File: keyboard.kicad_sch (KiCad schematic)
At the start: 27 parts, among them J1 USB_C_Receptacle_USB2.0_14P, SW1 SW_Push, SW2 SW_Push, SW3 SW_Push, SW4 SW_Push, SW5 SW_Push, U1 ATmega32U4-A, Y1 Crystal_GND24_Small

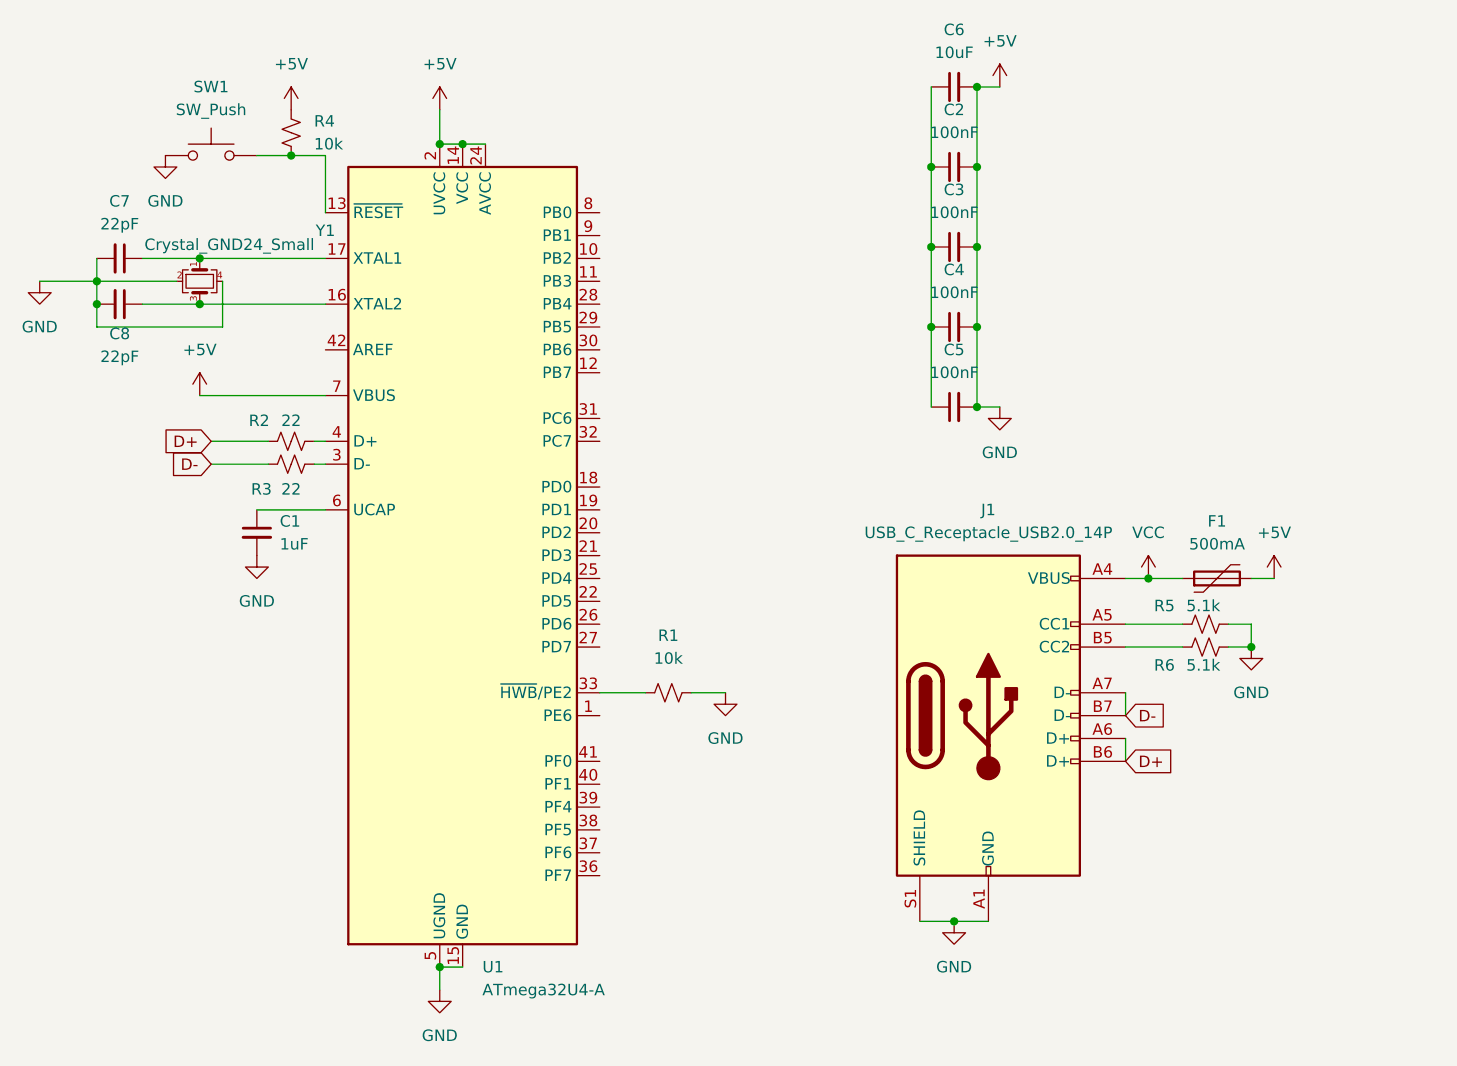
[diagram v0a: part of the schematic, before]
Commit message: bad
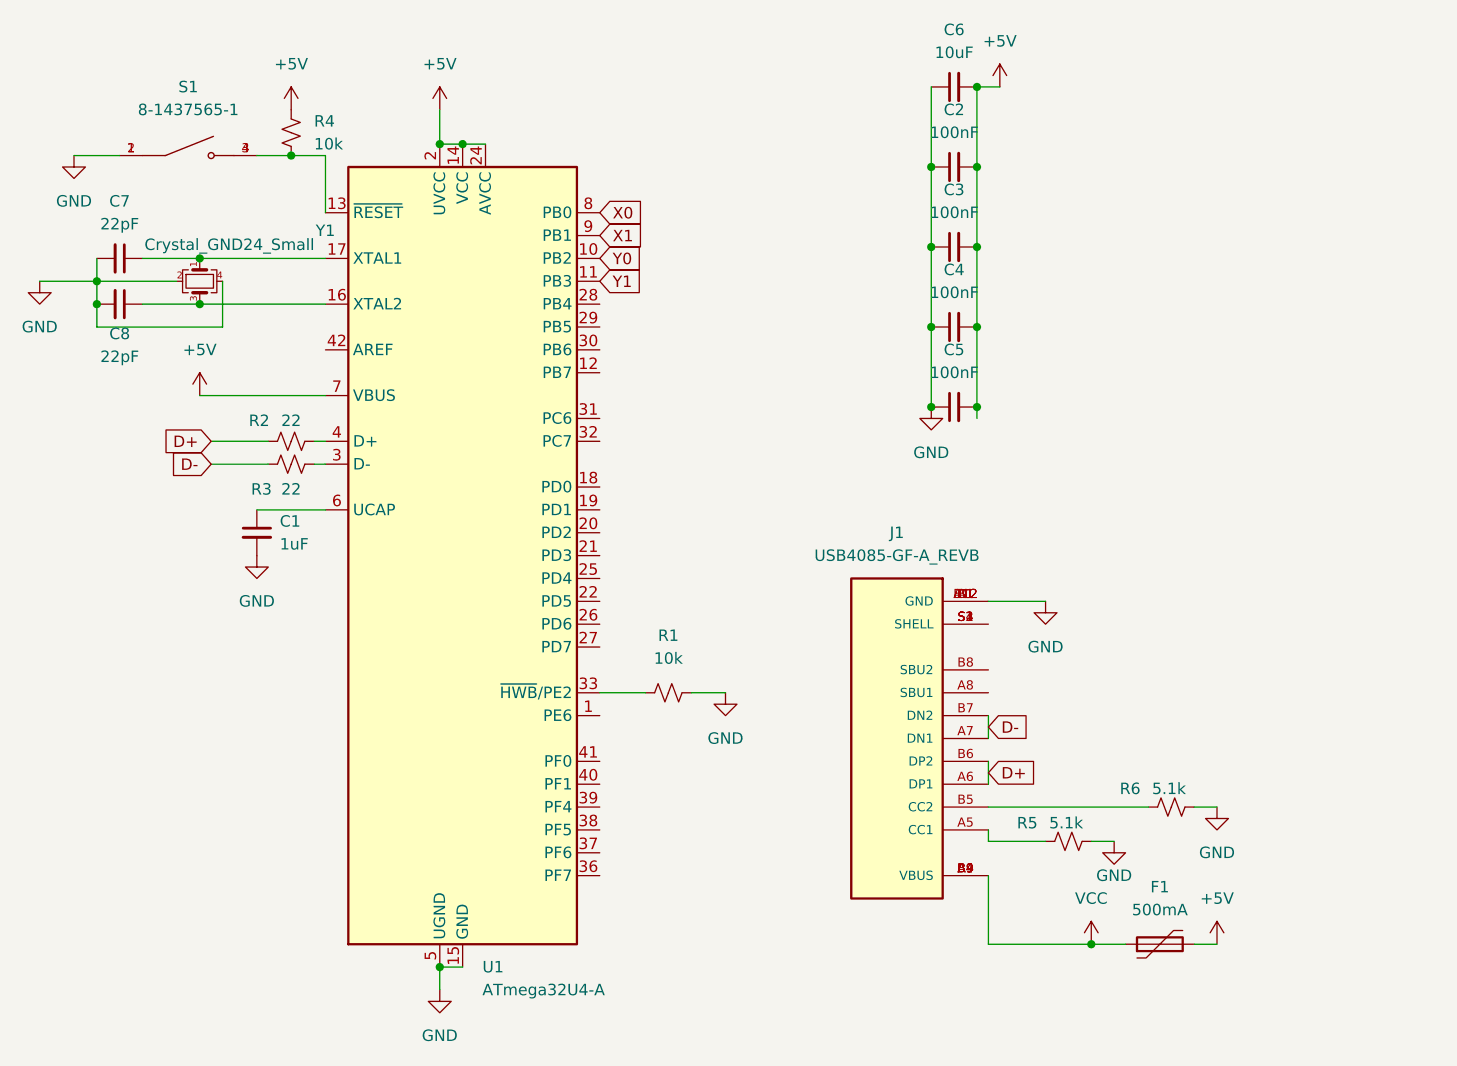
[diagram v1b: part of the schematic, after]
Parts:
- removed J1: USB_C_Receptacle_USB2.0_14P, symbol Connector:USB_C_Receptacle_USB2.0_14P
- removed SW1: SW_Push, symbol Switch:SW_Push
- added J1: USB4085-GF-A_REVB, USB-C:GCT_USB4085-GF-A_REVB, symbol USB4085-GF-A_REVB:USB4085-GF-A_REVB
- added S1: 8-1437565-1, Button:SW_8-1437565-1, symbol 8-1437565-1:8-1437565-1
- SW2, SW3, SW4, SW5: footprint (none) -> MX_keys:MX-Hotswap-1U
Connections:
- net +5V: no longer C1.2, C7.2, C8.2, R1.2, R5.2, R6.2, U1.15 (GND), U1.23 (GND), U1.35 (GND), U1.43 (GND), U1.5 (UGND), Y1.2, Y1.4
- net D+: now also J1.A6 (DP1), J1.B6 (DP2)
- net D-: now also J1.A7 (DN1), J1.B7 (DN2)
- net VCC: now also J1.A4 (VBUS), J1.A9 (VBUS), J1.B4 (VBUS), J1.B9 (VBUS)
- net X0: now also U1.8 (PB0)
- net X1: now also U1.9 (PB1)
- net Y0: now also U1.10 (PB2)
- net Y1: now also U1.11 (PB3)
- net at R4.2, U1.13 (~{RESET}): now also S1.3, S1.4
- net GND: now reaches C2.1, C3.1, C4.1, C5.1, C6.1
- net GND: now also C1.2, C7.2, C8.2, R1.2, R5.2, R6.2, U1.15 (GND), U1.23 (GND), U1.35 (GND), U1.43 (GND), U1.5 (UGND), Y1.2, Y1.4, J1.A1 (GND), J1.A12 (GND), J1.B1 (GND), J1.B12 (GND), S1.1, S1.2
- net at R6.1: now also J1.B5 (CC2)
- net at R5.1: now also J1.A5 (CC1)
- new net: J1.S1 (SHELL), J1.S2 (SHELL), J1.S3 (SHELL), J1.S4 (SHELL)

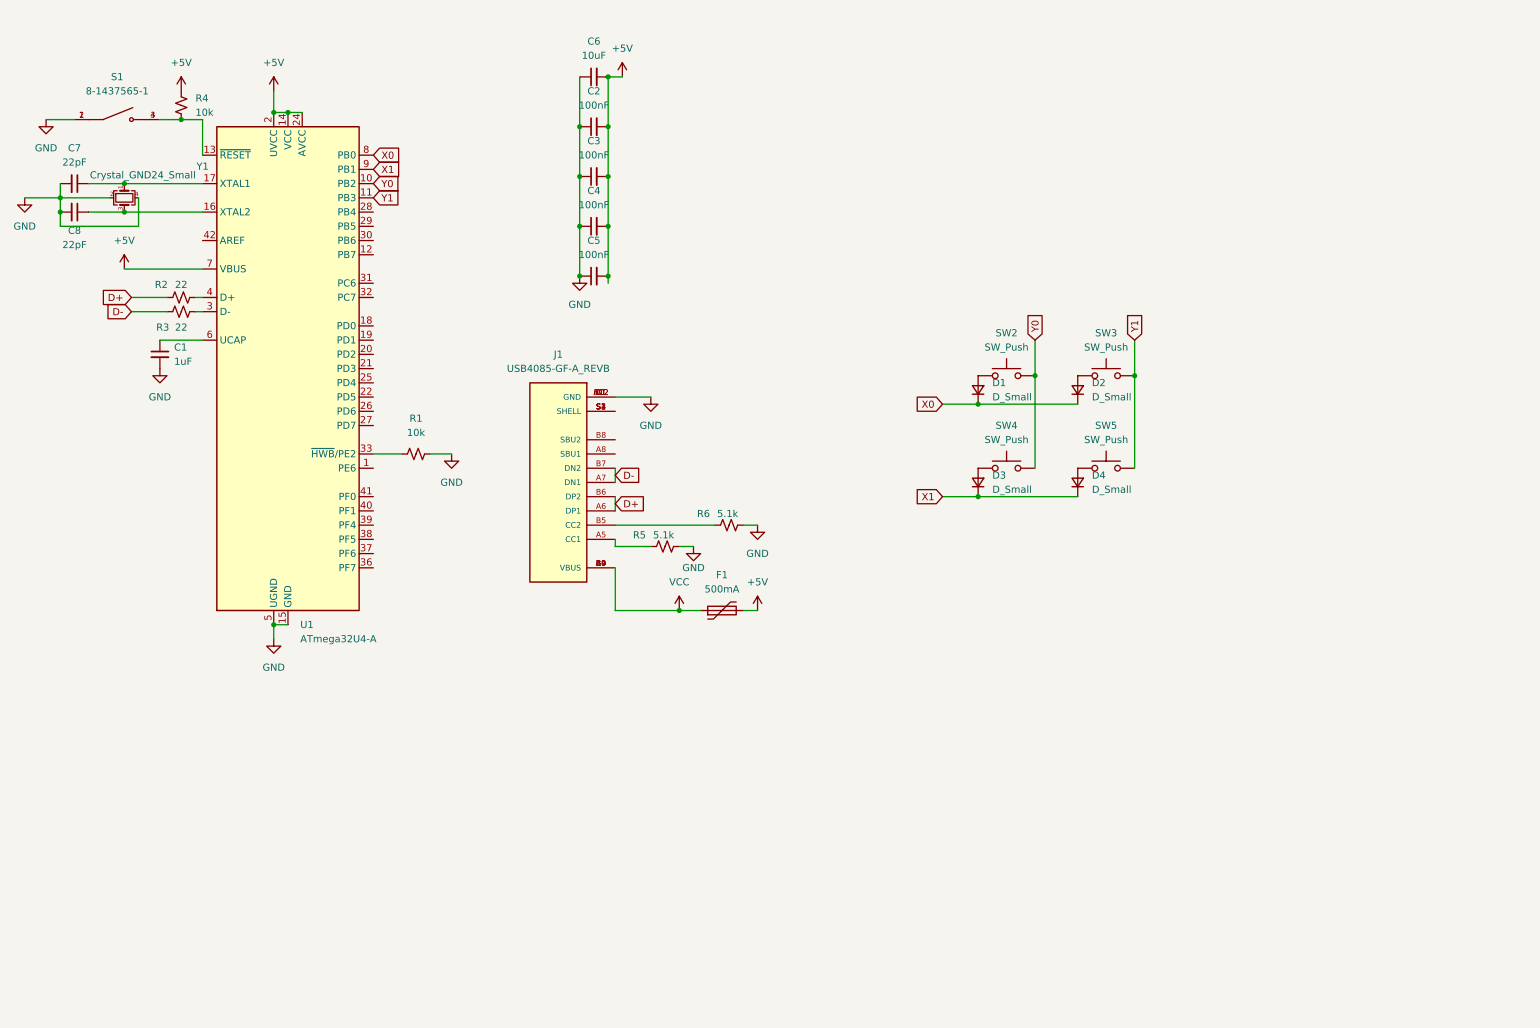
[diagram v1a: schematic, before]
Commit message: V1
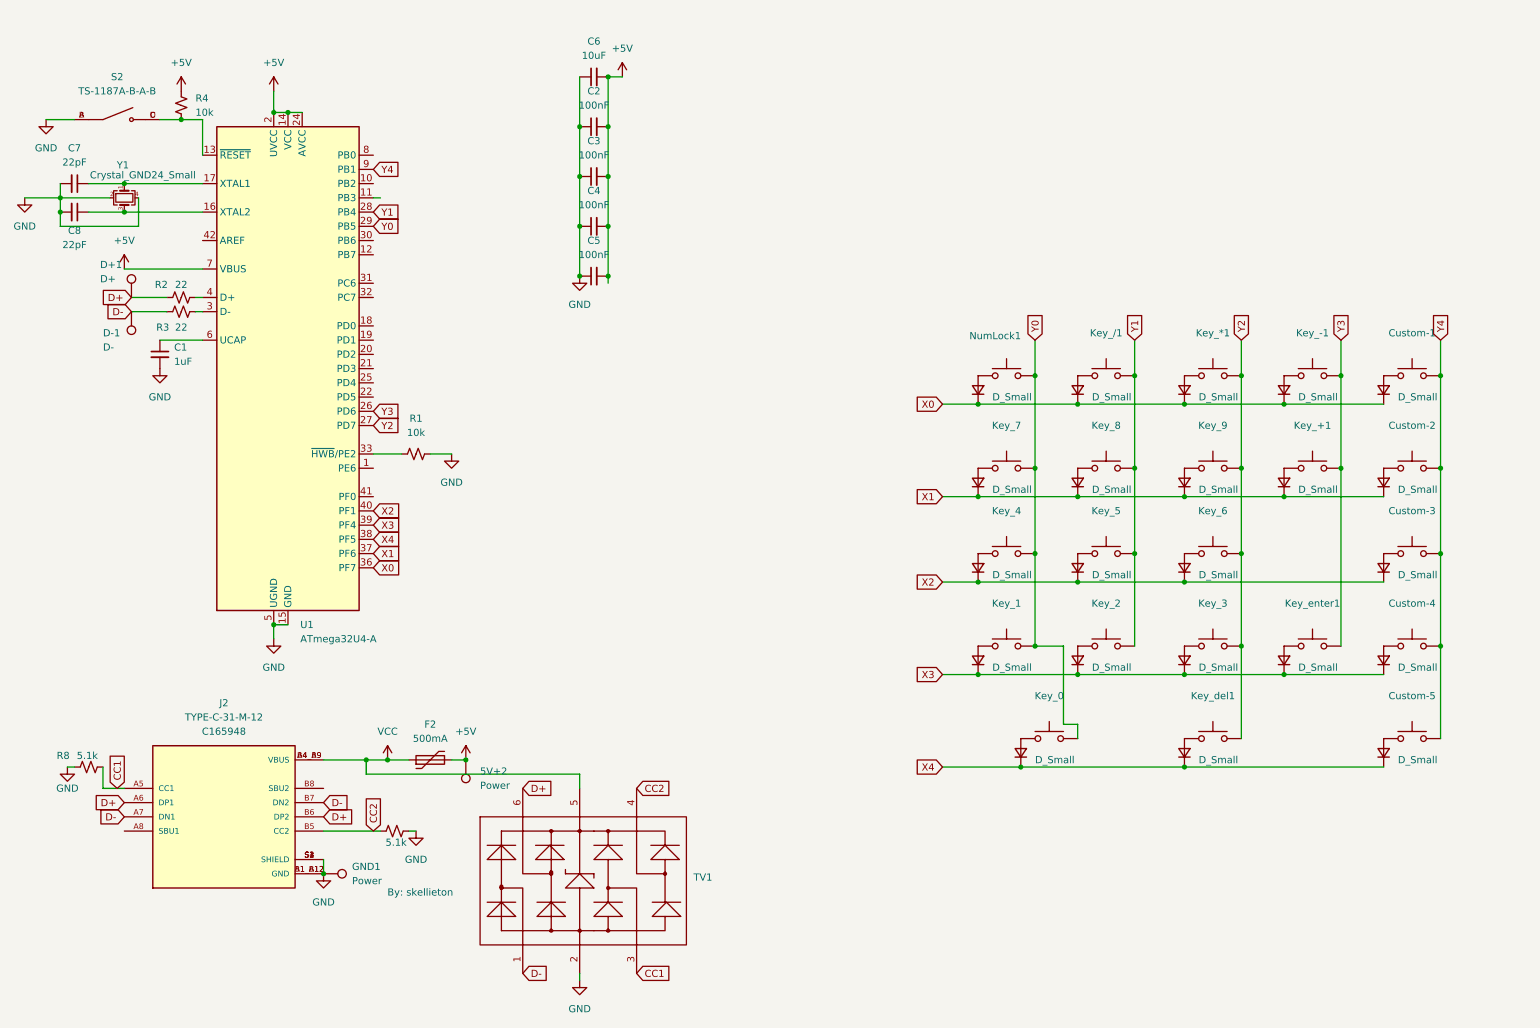
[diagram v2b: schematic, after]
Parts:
- removed F1: 500mA, Fuse:Fuse_1206_3216Metric, symbol Device:Polyfuse
- removed J1: USB4085-GF-A_REVB, USB-C:GCT_USB4085-GF-A_REVB, symbol USB4085-GF-A_REVB:USB4085-GF-A_REVB
- removed R5, R6: 5.1k, Resistor_SMD:R_0805_2012Metric, symbol Device:R_Small_US
- removed S1: 8-1437565-1, Button:SW_8-1437565-1, symbol 8-1437565-1:8-1437565-1
- added 5V+2, GND1: Power, TestPoint:TestPoint_Pad_1.0x1.0mm, symbol Connector:TestPoint
- added Custom-1, Custom-2, Custom-3, Custom-4, Custom-5, Key_*1, Key_-1, Key_1, Key_2, Key_3, Key_4, Key_5, Key_6, Key_9, Key_del1: SW_Push, MX_keys:MX-Hotswap-1U, symbol Switch:SW_Push
- added D+1: D+, TestPoint:TestPoint_Pad_1.0x1.0mm, symbol Connector:TestPoint
- added D-1: D-, TestPoint:TestPoint_Pad_1.0x1.0mm, symbol Connector:TestPoint
- added D10, D11, D12, D13, D14, D16, D17, D18, D19, D20, D21, D23, D25, D5, D6, D7, D8, D9: D_Small, Diode_SMD:D_SOD-123, symbol Device:D_Small
- added F2: 500mA, Fuse:Fuse_1206_3216Metric, symbol Device:Polyfuse
- added J2: TYPE-C-31-M-12, USB-C:HRO_TYPE-C-31-M-12, symbol MyLib:TYPE-C-31-M-12
- added Key_+1, Key_enter1: SW_Push_U2, Button_Switch_Keyboard:MX-Hotswap-2U-Vertical-ReversedStabilizers, symbol Switch:SW_Push
- added Key_0: SW_Push_U2, Button_Switch_Keyboard:MX-Hotswap-2U-ReversedStabilizers, symbol Switch:SW_Push
- added R7, R8: 5.1k, Resistor_SMD:R_0805_2012Metric, symbol Device:R_Small_US
- added S2: TS-1187A-B-A-B, USB-C:SW_TS-1187A-B-A-B, symbol MyLib:TS-1187A-B-A-B
- added TV1: ~, Button_Switch_Keyboard:SOT-23-6_L2.9-W1.6-P0.95-LS2.8-BR, symbol MyLib:SRV05-4-P-T7
- C1: LCSC (none) -> C28323
- C2, C3, C4: LCSC (none) -> C49678
- C5: LSCS (none) -> C49678
- C6: LCSC (none) -> C15850
- C7: LCSC (none) -> C1804
- C8: LSCS (none) -> C1804
- D1, D2: LCSC (none) -> C64898
- NumLock1: renamed from SW2; LCSC (none) -> C41430893
- R1, R4: LCSC (none) -> C17414
- R2, R3: LCSC (none) -> C17561
- Y1: LCSC (none) -> C13738
- renumbered SW3 to Key_/1, SW4 to Key_7, SW5 to Key_8
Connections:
- net +5V: now also 5V+2.1, F2.2
- net D+: now also D+1.1, J2.A6 (DP1), J2.B6 (DP2), TV1.6
- net D-: now also D-1.1, J2.A7 (DN1), J2.B7 (DN2), TV1.1
- net GND: now also GND1.1, J2.A1_B12 (GND), J2.B1_A12 (GND), J2.S1 (SHIELD), J2.S2 (SHIELD), J2.S3 (SHIELD), J2.S4 (SHIELD), R7.1, R8.1, S2.A, S2.B, TV1.2
- net VCC: now also F2.1, J2.A4_B9 (VBUS), J2.B4_A9 (VBUS), TV1.5
- net X0: now also U1.36 (PF7), D11.1 (K), D17.1 (K), D9.1 (K); no longer U1.8 (PB0)
- net X1: now also U1.37 (PF6), D10.1 (K), D12.1 (K), D18.1 (K); no longer U1.9 (PB1)
- net Y0: now also U1.29 (PB5), Key_0.2, Key_1.2, Key_4.2; no longer U1.10 (PB2)
- net Y1: now also U1.28 (PB4), Key_2.2, Key_5.2; no longer U1.11 (PB3)
- net at R4.2, U1.13 (~{RESET}): now also S2.C, S2.D
- net Y3: now reaches U1.26 (PD6)
- net Y3: now also Key_+1.2, Key_-1.2, Key_enter1.2
- net Y2: now reaches U1.27 (PD7)
- net Y2: now also Key_*1.2, Key_3.2, Key_6.2, Key_9.2, Key_del1.2
- net X4: now reaches U1.38 (PF5)
- net X4: now also D21.1 (K), D23.1 (K), D25.1 (K)
- net X3: now reaches U1.39 (PF4)
- net X3: now also D14.1 (K), D16.1 (K), D20.1 (K), D6.1 (K), D8.1 (K)
- net X2: now reaches U1.40 (PF1)
- net X2: now also D13.1 (K), D19.1 (K), D5.1 (K), D7.1 (K)
- new net: D12.2 (A), Key_+1.1
- new net: D14.2 (A), Key_3.1
- new net: D11.2 (A), Key_-1.1
- new net: Custom-3.1, D19.2 (A)
- new net: D21.2 (A), Key_0.1
- new net: D16.2 (A), Key_enter1.1
- new net: D10.2 (A), Key_9.1
- new net: Custom-5.1, D25.2 (A)
- new net: D7.2 (A), Key_5.1
- new net: D6.2 (A), Key_1.1
- new net: D23.2 (A), Key_del1.1
- new net: D8.2 (A), Key_2.1
- new net: Custom-4.1, D20.2 (A)
- new net: Custom-2.1, D18.2 (A)
- new net: Custom-1.1, D17.2 (A)
- new net: D9.2 (A), Key_*1.1
- new net: D5.2 (A), Key_4.1
- new net: D13.2 (A), Key_6.1
- new net CC1: J2.A5 (CC1), R8.2, TV1.3
- new net CC2: J2.B5 (CC2), R7.2, TV1.4
- new net Y4: Custom-1.2, Custom-2.2, Custom-3.2, Custom-4.2, Custom-5.2, U1.9 (PB1)
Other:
- note added: "By: skellieton"

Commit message: fixFlip
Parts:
- Key_+1, Key_enter1: footprint Button_Switch_Keyboard:MX-Hotswap-2U-Vertical-ReversedStabilizers -> Button_Switch_Keyboard:MX-Hotswap-2U-ReversedStabilizers
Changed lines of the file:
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@@
 			)
 		)
-		(property "Footprint" "Button_Switch_Keyboard:MX-Hotswap-2U-Vertical-ReversedStabilizers"
+		(property "Footprint" "Button_Switch_Keyboard:MX-Hotswap-2U-ReversedStabilizers"
 			(at 246.38 88.9 0)
 			(effects
@@
 			)
 		)
-		(property "Footprint" "Button_Switch_Keyboard:MX-Hotswap-2U-Vertical-ReversedStabilizers"
+		(property "Footprint" "Button_Switch_Keyboard:MX-Hotswap-2U-ReversedStabilizers"
 			(at 246.38 120.65 0)
 			(effects
